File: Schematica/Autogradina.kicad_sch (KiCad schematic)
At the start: 39 parts, among them IC1 NodeMCU, J1 Priza Pompa, K1 CONTACTOR, P1 Conector putere, P2 Conector periferice 220V, Q1 BC547, Q2 BC547, Q3 BC547, Q4 IRLZ44N, Q5 IRLZ44N, Q6 IRLZ44N, Q7 IRLZ44N, Q8 IRLZ44N

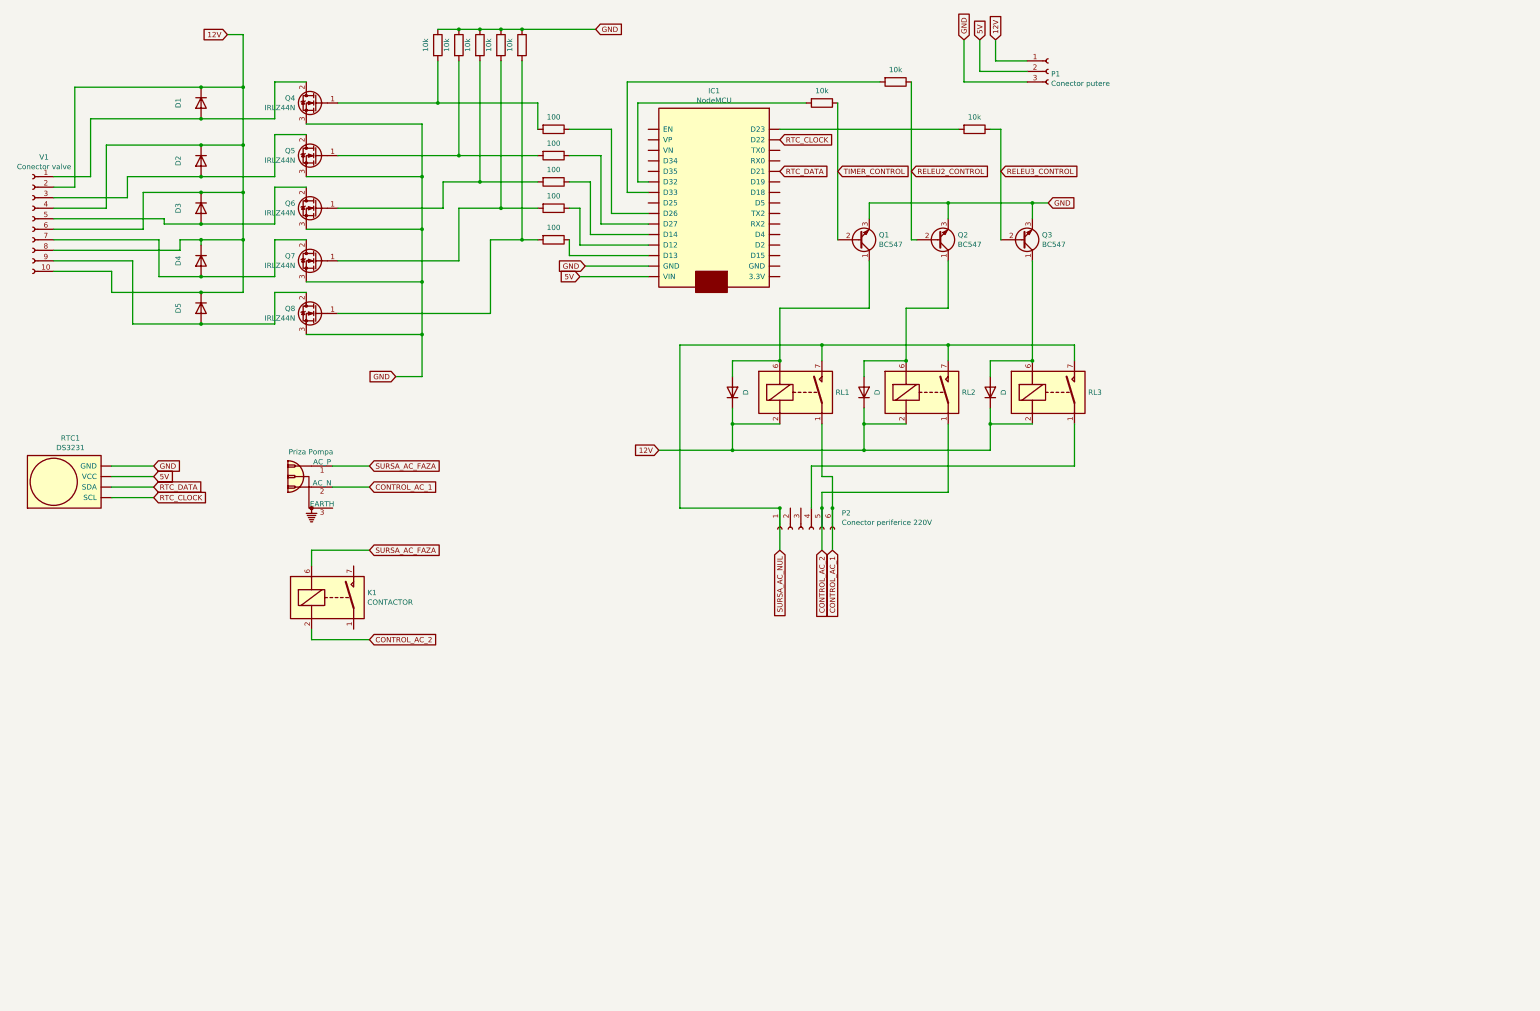
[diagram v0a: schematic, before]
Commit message: Schematic updates; Created board
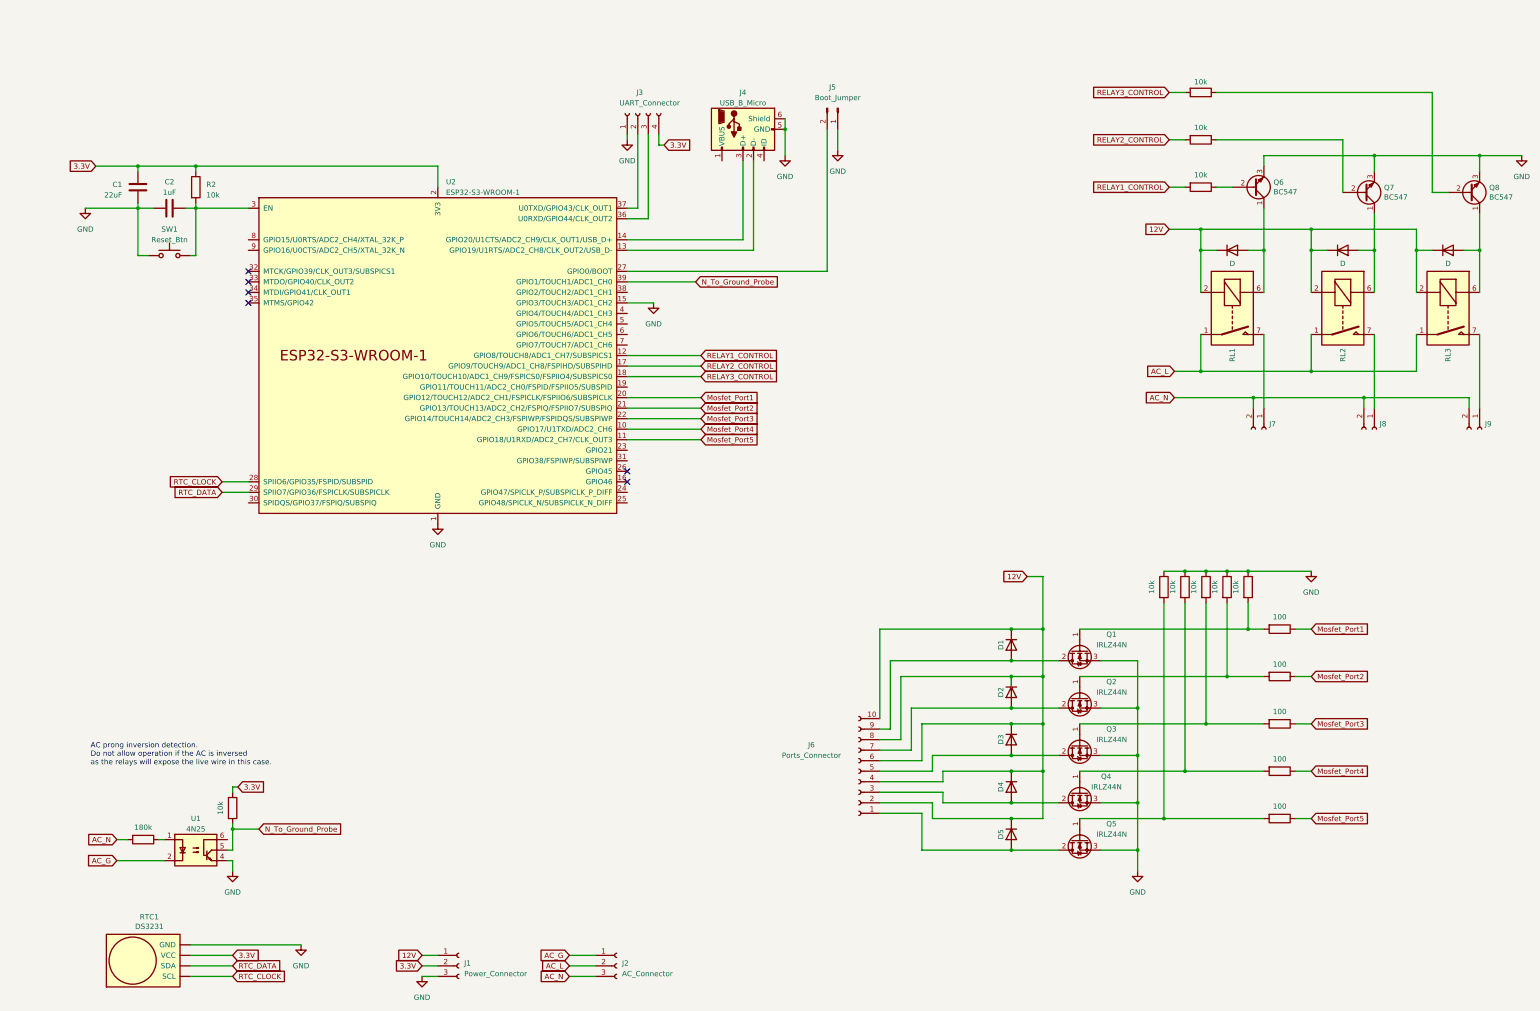
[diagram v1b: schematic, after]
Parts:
- removed IC1: NodeMCU, symbol Custom:NodeMCU
- removed J1: Priza Pompa, symbol Connector:Conn_WallSocket_Earth
- removed K1: CONTACTOR, Relay_THT:Relay_StandexMeder_DIP_LowProfile, symbol Relay:DIPxx-1Axx-11x
- removed P1: Conector putere, symbol Connector:Conn_01x03_Female
- removed P2: Conector periferice 220V, symbol Connector:Conn_01x06_Female
- removed V1: Conector valve, symbol Connector:Conn_01x10_Female
- added C1: 22uF, Capacitor_THT:CP_Radial_D6.3mm_P2.50mm, symbol Device:C
- added C2: 1uF, Capacitor_THT:CP_Radial_D6.3mm_P2.50mm, symbol Device:C
- added J1: Power_Connector, Custom:Connector_RND_205-00113_3Pins_3.5mm, symbol Connector:Conn_01x03_Socket
- added J2: AC_Connector, Custom:Connector_RND_205-00113_3Pins_3.5mm, symbol Connector:Conn_01x03_Socket
- added J3: UART_Connector, Connector_PinSocket_2.54mm:PinSocket_1x04_P2.54mm_Vertical, symbol Connector:Conn_01x04_Socket
- added J4: USB_B_Micro, Connector_USB:USB_Micro-B_Wuerth_629105150521, symbol Connector:USB_B_Micro
- added J5: Boot_Jumper, Connector_PinHeader_2.54mm:PinHeader_1x02_P2.54mm_Vertical, symbol Connector:Conn_01x02_Pin
- added J6: Ports_Connector, Custom:Connector_Wire-To-Board_10Pins_2.54mm, symbol Connector:Conn_01x10_Socket
- added J7, J8, J9: Conn_01x02_Socket, Custom:Connector_RND_205-00113_2Pins_3.5mm, symbol Connector:Conn_01x02_Socket
- added R1: 180k, Resistor_THT:R_Axial_DIN0207_L6.3mm_D2.5mm_P10.16mm_Horizontal, symbol Device:R
- added R2, R3: 10k, Resistor_THT:R_Axial_DIN0207_L6.3mm_D2.5mm_P10.16mm_Horizontal, symbol Device:R
- added SW1: Reset_Btn, Button_Switch_THT:SW_PUSH_6mm, symbol Switch:SW_Push
- added U1: 4N25, Package_DIP:DIP-6_W7.62mm, symbol Isolator:4N25
- added U2: ESP32-S3-WROOM-1, Expressif:ESP32-S3-WROOM-1U, symbol Expressif:ESP32-S3-WROOM-1
- D1, D2, D3, D4, D5, D6, D7, D8: footprint (none) -> Diode:1N4007
- R10: renamed from R4; footprint (none) -> Resistor_THT:R_Axial_DIN0207_L6.3mm_D2.5mm_P10.16mm_Horizontal
- R11: renamed from R5; footprint (none) -> Resistor_THT:R_Axial_DIN0207_L6.3mm_D2.5mm_P10.16mm_Horizontal
- R12: renamed from R6; footprint (none) -> Resistor_THT:R_Axial_DIN0207_L6.3mm_D2.5mm_P10.16mm_Horizontal
- R13: renamed from R7; footprint (none) -> Resistor_THT:R_Axial_DIN0207_L6.3mm_D2.5mm_P10.16mm_Horizontal
- R14: renamed from R8; footprint (none) -> Resistor_THT:R_Axial_DIN0207_L6.3mm_D2.5mm_P10.16mm_Horizontal
- R15: renamed from R9; footprint (none) -> Resistor_THT:R_Axial_DIN0207_L6.3mm_D2.5mm_P10.16mm_Horizontal
- R16: renamed from R10; footprint (none) -> Resistor_THT:R_Axial_DIN0207_L6.3mm_D2.5mm_P10.16mm_Horizontal
- R4: renamed from R1; footprint (none) -> Resistor_THT:R_Axial_DIN0207_L6.3mm_D2.5mm_P10.16mm_Horizontal
- R5: renamed from R2; footprint (none) -> Resistor_THT:R_Axial_DIN0207_L6.3mm_D2.5mm_P10.16mm_Horizontal
- R6: renamed from R13; footprint (none) -> Resistor_THT:R_Axial_DIN0207_L6.3mm_D2.5mm_P10.16mm_Horizontal
- R7: renamed from R12; footprint (none) -> Resistor_THT:R_Axial_DIN0207_L6.3mm_D2.5mm_P10.16mm_Horizontal
- R8: renamed from R11; footprint (none) -> Resistor_THT:R_Axial_DIN0207_L6.3mm_D2.5mm_P10.16mm_Horizontal
- R9: renamed from R3; footprint (none) -> Resistor_THT:R_Axial_DIN0207_L6.3mm_D2.5mm_P10.16mm_Horizontal
- RTC1: footprint (none) -> Custom:RTC-Module
- renumbered Q4 to Q1, Q5 to Q2, Q6 to Q3, Q7 to Q4, Q8 to Q5, Q1 to Q6, Q2 to Q7, Q3 to Q8
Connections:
- net CONTROL_AC_1 is gone; now on net AC_L: RL1.1, RL1.14
- net CONTROL_AC_2 is gone; now on net AC_L: RL2.1, RL2.14
- net 12V: now also J1.1 (Pin_1), J6.10 (Pin_10), J6.2 (Pin_2), J6.4 (Pin_4), J6.6 (Pin_6), J6.8 (Pin_8)
- net GND: now also C1.2, C2.1, J1.3 (Pin_3), J3.1 (Pin_1), J4.5 (GND), J4.6 (Shield), J5.1 (Pin_1), SW1.1, U1.4, U2.1 (GND), U2.15 (GPIO3/TOUCH3/ADC1_CH2), U2.40 (GND), U2.41 (GND)
- net RTC_CLOCK: now also U2.28 (SPIIO6/GPIO35/FSPID/SUBSPID)
- net RTC_DATA: now also U2.29 (SPIIO7/GPIO36/FSPICLK/SUBSPICLK)
- net at Q1.1 (G), R12.2: now also R11.2; no longer R4.2
- net at D1.2 (A), Q1.2 (D): now also J6.9 (Pin_9)
- net at Q2.1 (G), R13.2: now also R10.2; no longer R5.2
- net at D2.2 (A), Q2.2 (D): now also J6.7 (Pin_7)
- net at D3.2 (A), Q3.2 (D): now also J6.5 (Pin_5)
- net at Q4.1 (G), R15.2: now also R5.2; no longer R10.2
- net at D4.2 (A), Q4.2 (D): now also J6.3 (Pin_3)
- net at Q5.1 (G), R16.2: now also R4.2; no longer R11.2
- net at D5.2 (A), Q5.2 (D): now also J6.1 (Pin_1)
- net RELAY2_CONTROL: now reaches R7.2
- net RELAY2_CONTROL: now also U2.17 (GPIO9/TOUCH9/ADC1_CH8/FSPIHD/SUBSPIHD)
- net RELAY1_CONTROL: now reaches R8.2
- net RELAY1_CONTROL: now also U2.12 (GPIO8/TOUCH8/ADC1_CH7/SUBSPICS1)
- net Mosfet_Port2: now reaches R13.1
- net Mosfet_Port2: now also U2.21 (GPIO13/TOUCH13/ADC2_CH2/FSPIQ/FSPIIO7/SUBSPIQ)
- net Mosfet_Port1: now reaches R12.1
- net Mosfet_Port1: now also U2.20 (GPIO12/TOUCH12/ADC2_CH1/FSPICLK/FSPIIO6/SUBSPICLK)
- net RELAY3_CONTROL: now reaches R6.2
- net RELAY3_CONTROL: now also U2.18 (GPIO10/TOUCH10/ADC1_CH9/FSPICS0/FSPIIO4/SUBSPICS0)
- net Mosfet_Port3: now reaches R14.1
- net Mosfet_Port3: now also U2.22 (GPIO14/TOUCH14/ADC2_CH3/FSPIWP/FSPIDQS/SUBSPIWP)
- net Mosfet_Port5: now reaches R16.1
- net Mosfet_Port5: now also U2.11 (GPIO18/U1RXD/ADC2_CH7/CLK_OUT3)
- net Mosfet_Port4: now reaches R15.1
- net Mosfet_Port4: now also U2.10 (GPIO17/U1TXD/ADC2_CH6)
- net AC_L: now reaches RL3.1, RL3.14
- net AC_L: now also J2.2 (Pin_2)
- net 5V renamed 3.3V
- net 3.3V: now also C1.1, J1.2 (Pin_2), J3.4 (Pin_4), R2.1, R3.1, U2.2 (3V3)
- net RELEU2_CONTROL: no longer names the net of Q7.2 (B), R7.1
- net RELEU3_CONTROL: no longer names the net of Q8.2 (B), R6.1
- removed net SURSA_AC_NUL: RL1.7, RL1.8, RL2.7, RL2.8, RL3.7, RL3.8
- net TIMER_CONTROL: no longer names the net of Q6.2 (B), R8.1
- new net: J7.1 (Pin_1), RL1.7, RL1.8
- new net: J8.1 (Pin_1), RL2.7, RL2.8
- new net: J9.1 (Pin_1), RL3.7, RL3.8
- new net: J3.2 (Pin_2), U2.37 (U0TXD/GPIO43/CLK_OUT1)
- new net: J3.3 (Pin_3), U2.36 (U0RXD/GPIO44/CLK_OUT2)
- new net: R1.1, U1.1
- new net: J5.2 (Pin_2), U2.27 (GPIO0/BOOT)
- new net: C2.2, R2.2, SW1.2, U2.3 (EN)
- new net: J4.2 (D-), U2.13 (GPIO19/U1RTS/ADC2_CH8/CLK_OUT2/USB_D-)
- new net: J4.3 (D+), U2.14 (GPIO20/U1CTS/ADC2_CH9/CLK_OUT1/USB_D+)
- new net AC_G: J2.1 (Pin_1), U1.2
- new net AC_N: J2.3 (Pin_3), J7.2 (Pin_2), J8.2 (Pin_2), J9.2 (Pin_2), R1.2
- new net N_To_Ground_Probe: R3.2, U1.5, U2.39 (GPIO1/TOUCH1/ADC1_CH0)
- no-connect marks 0 -> 6
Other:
- note added: "AC prong inversion detection. Do not allow operation if the AC is inversed as the relays will expose the live wire in this case."
- moved on the sheet: D1, D2, D3, D4, D5, Q1, Q2, Q3, Q4, Q5, Q6, Q7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
